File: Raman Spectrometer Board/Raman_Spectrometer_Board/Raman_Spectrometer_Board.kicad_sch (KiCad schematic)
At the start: 37 parts, among them J1 RJ45_LED_Shielded, Q1 BSS138, Q2 BSS138, Q3 BSS138, Q4 BSS138, SW1 SW_Push, SW2 SW_Push, U1 Teensy4.1_DEV-16771, U2 OKI 12V-5V

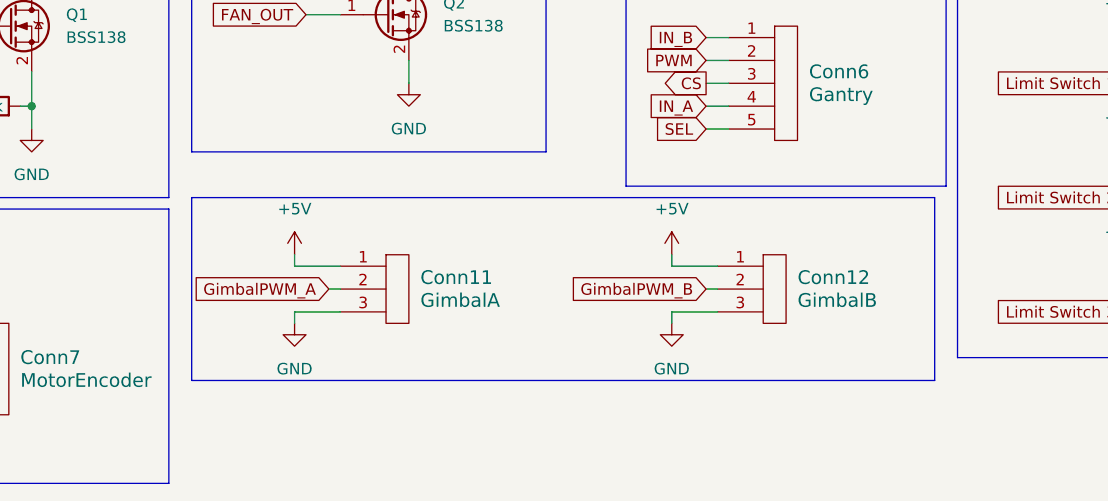
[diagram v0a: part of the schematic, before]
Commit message: Finished Rev2
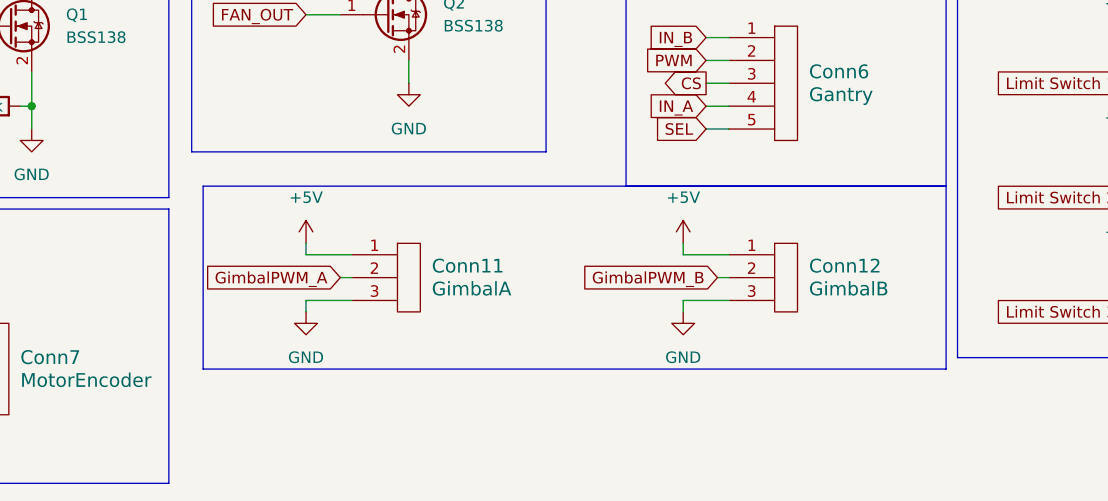
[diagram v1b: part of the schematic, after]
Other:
- moved on the sheet: Conn11, Conn12
